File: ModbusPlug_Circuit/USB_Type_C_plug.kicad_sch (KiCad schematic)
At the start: 6 parts, among them P1 USB_C_Plug, U1 MCP1700x-330xxTT, U4 USBLC6-2SC6

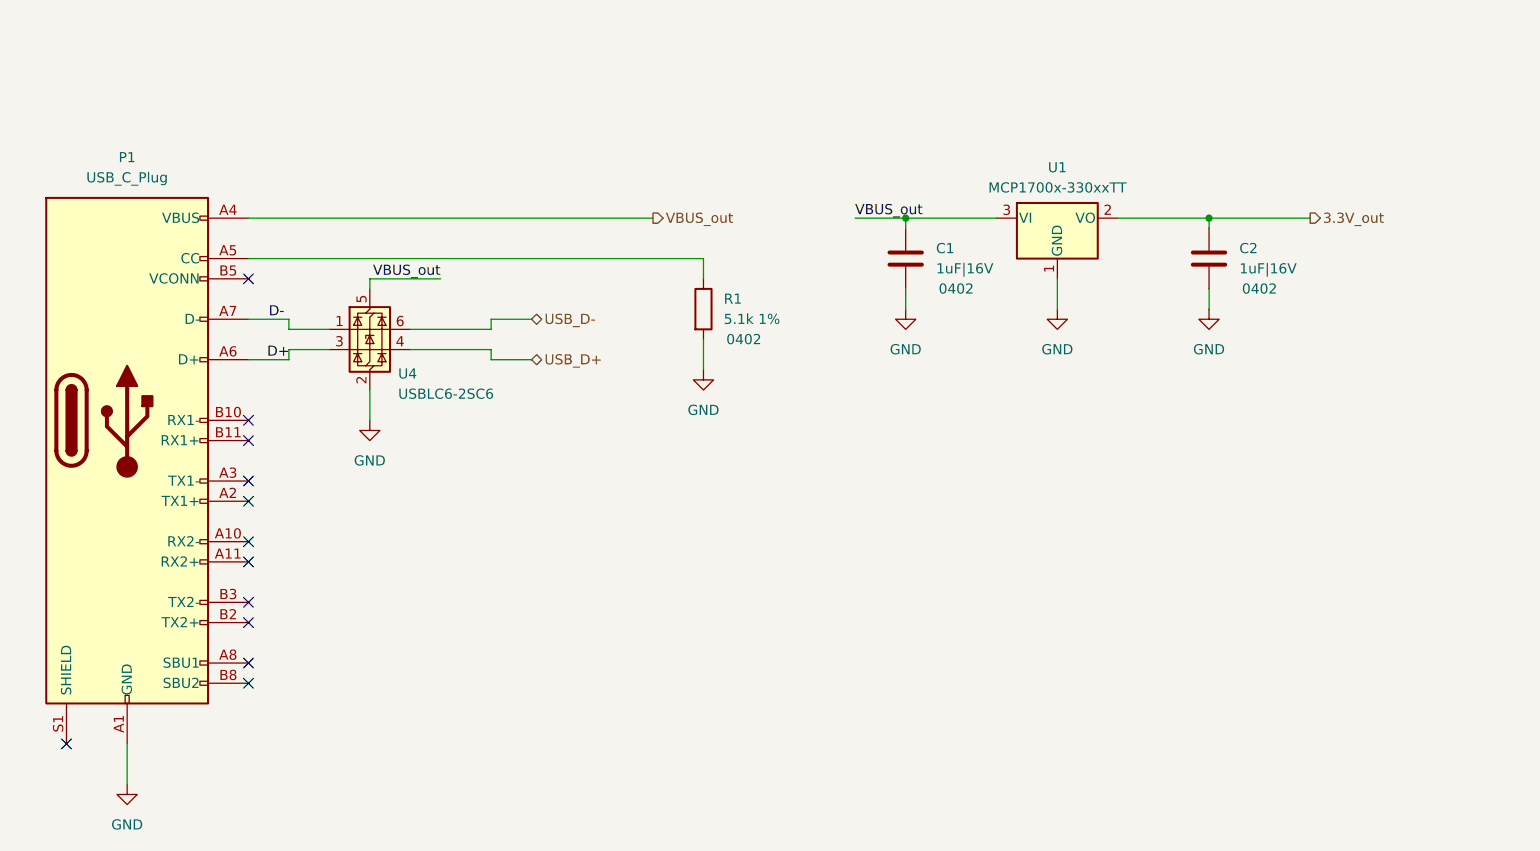
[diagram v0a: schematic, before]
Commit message: pushing V0.1.4
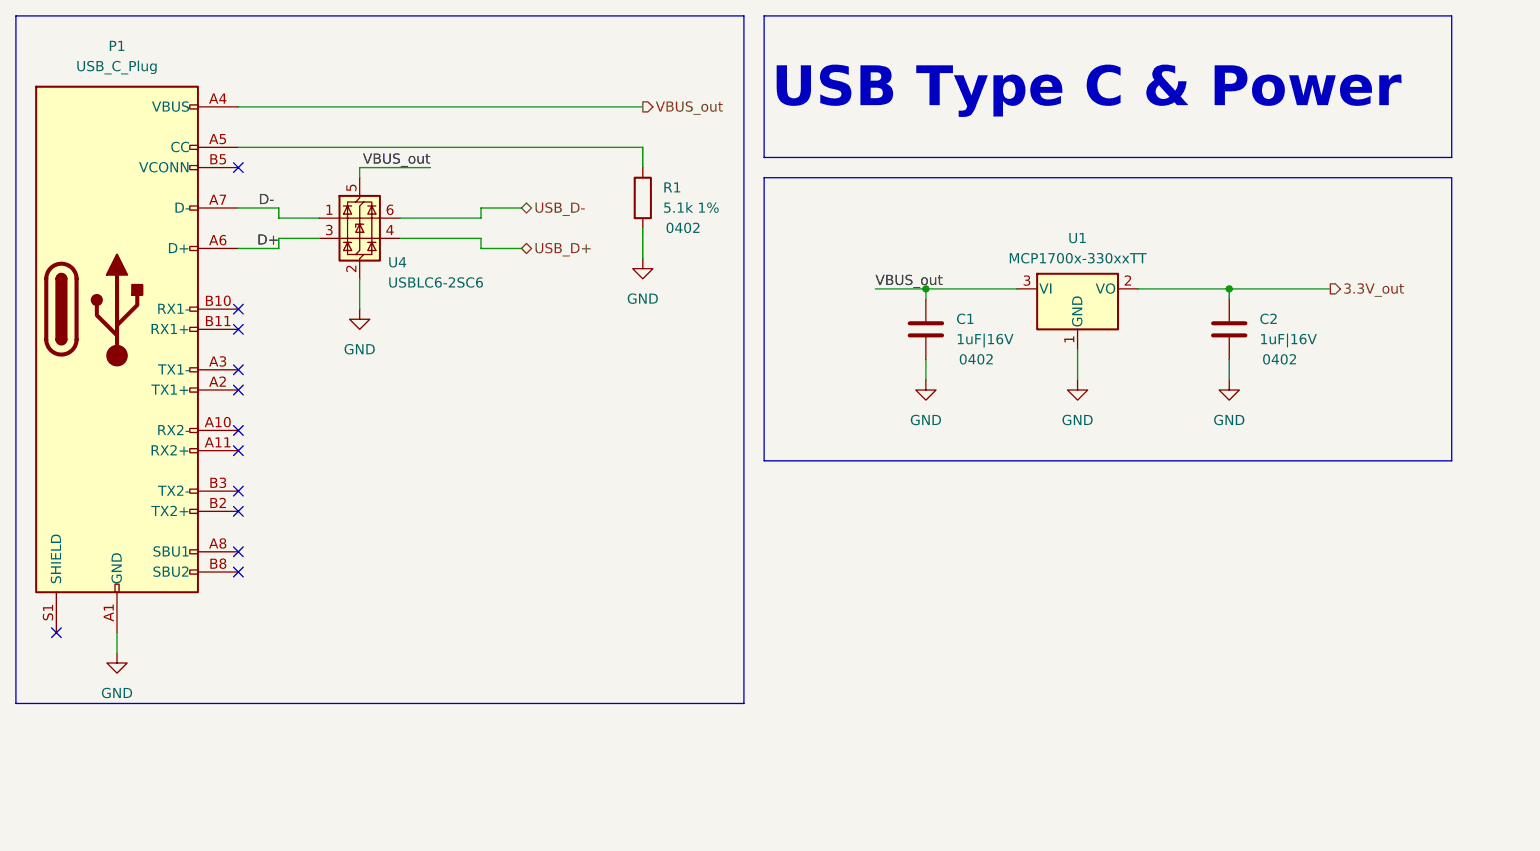
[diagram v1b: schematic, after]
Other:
- title: (none) -> ModbusPlug
- moved on the sheet: C1, C2, P1, R1, U1, U4
